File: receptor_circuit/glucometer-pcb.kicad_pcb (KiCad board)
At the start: 2 copper layers, 43.3 x 60.7 mm, 19 parts, among them IC1 RC4558IP, IC2 LM1458N, IC3 RC4558IP

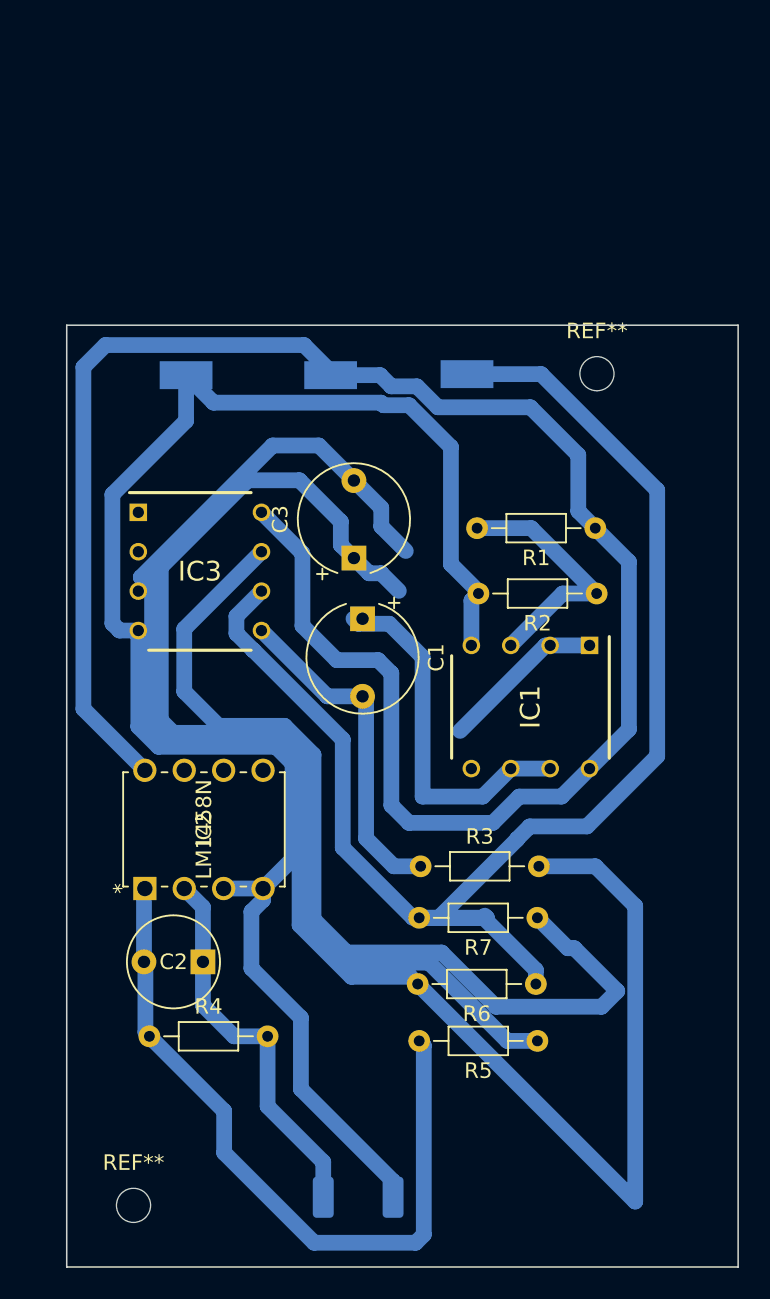
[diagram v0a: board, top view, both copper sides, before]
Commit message: last update reciver circuit pcb
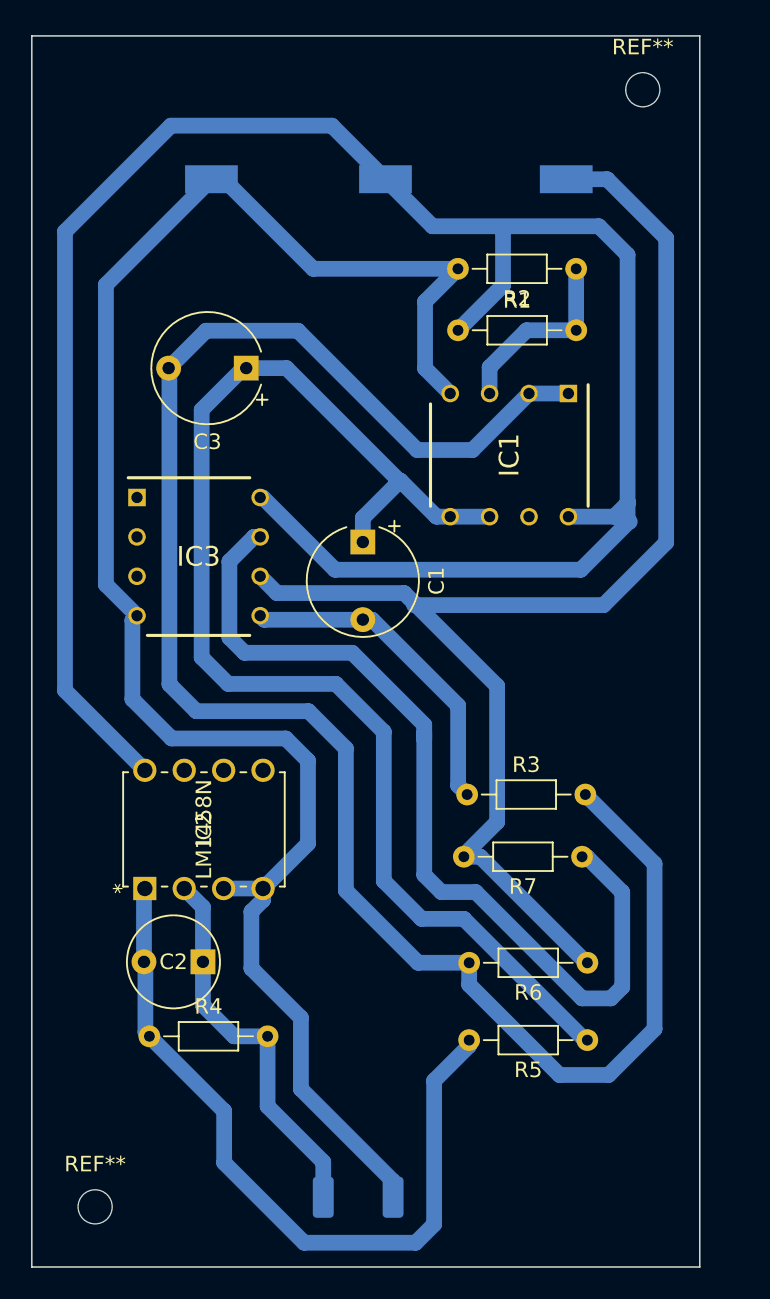
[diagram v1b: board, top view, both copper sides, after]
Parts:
- moved R2 21.0 mm to (205.6, 115.0)
- moved REF** 18.5 mm to (209.9, 103.5)
- moved IC1 16.3 mm to (201.3, 127.0)
- moved R1 15.5 mm to (198.0, 119.0), turned to 0 degrees
- moved TP3 14.1 mm to (205.0, 109.2)
- moved C3 14.1 mm to (184.3, 121.4), turned to 180 degrees
- moved TP2 13.1 mm to (193.3, 109.2)
- moved TP1 12.7 mm to (182.1, 109.2)
- moved R3 5.51 mm to (198.6, 148.9)
- moved C1 4.95 mm to (191.9, 132.6)
- moved R7 4.88 mm to (206.0, 152.9)
- moved R6 3.59 mm to (206.3, 159.7)
- moved R5 3.22 mm to (206.3, 164.7)
- moved REF** 2.48 mm to (174.6, 175.5)
- moved IC3 0.96 mm to (181.3, 133.5)
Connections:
- C1 pad 1: Net-(C1-Pad1) -> /SIGNAL_1
- IC1 pad 6: Net-(C1-Pad1) -> /SIGNAL_1
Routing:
- net Net-(C1-Pad1): track 23.4 -> 0.00 mm
- net /SIGNAL_1: track 70.4 -> 85.2 mm
- net VCC: track 124.4 -> 135.6 mm
- net GND: track 105.0 -> 113.5 mm
- net Net-(IC3-Pad6): track 93.4 -> 86.4 mm
- net Net-(IC1-Pad3): track 16.4 -> 12.2 mm
- net /PWD_1.65: track 121.7 -> 118.1 mm
- net Net-(IC3-Pad7): track 61.2 -> 58.6 mm
- net Net-(C2-Pad2): track 47.3 -> 48.8 mm
- net /SIGNAL_2: track 21.9 -> 21.1 mm
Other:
- board size 43.3 x 60.7 mm -> 43.1 x 79.4 mm
